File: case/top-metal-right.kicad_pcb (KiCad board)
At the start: 2 copper layers, 135 x 93.7 mm, 26 parts, among them SW1 SW_PUSH, SW10 SW_PUSH, SW11 SW_PUSH, SW12 SW_PUSH, SW13 SW_PUSH, SW14 SW_PUSH, SW15 SW_PUSH, SW16 SW_PUSH, SW17 SW_PUSH, SW18 SW_PUSH, SW19 SW_PUSH, SW2 SW_PUSH, SW20 SW_PUSH, SW3 SW_PUSH, SW4 SW_PUSH, SW5 SW_PUSH, SW6 SW_PUSH, SW7 SW_PUSH, SW8 SW_PUSH, SW9 SW_PUSH

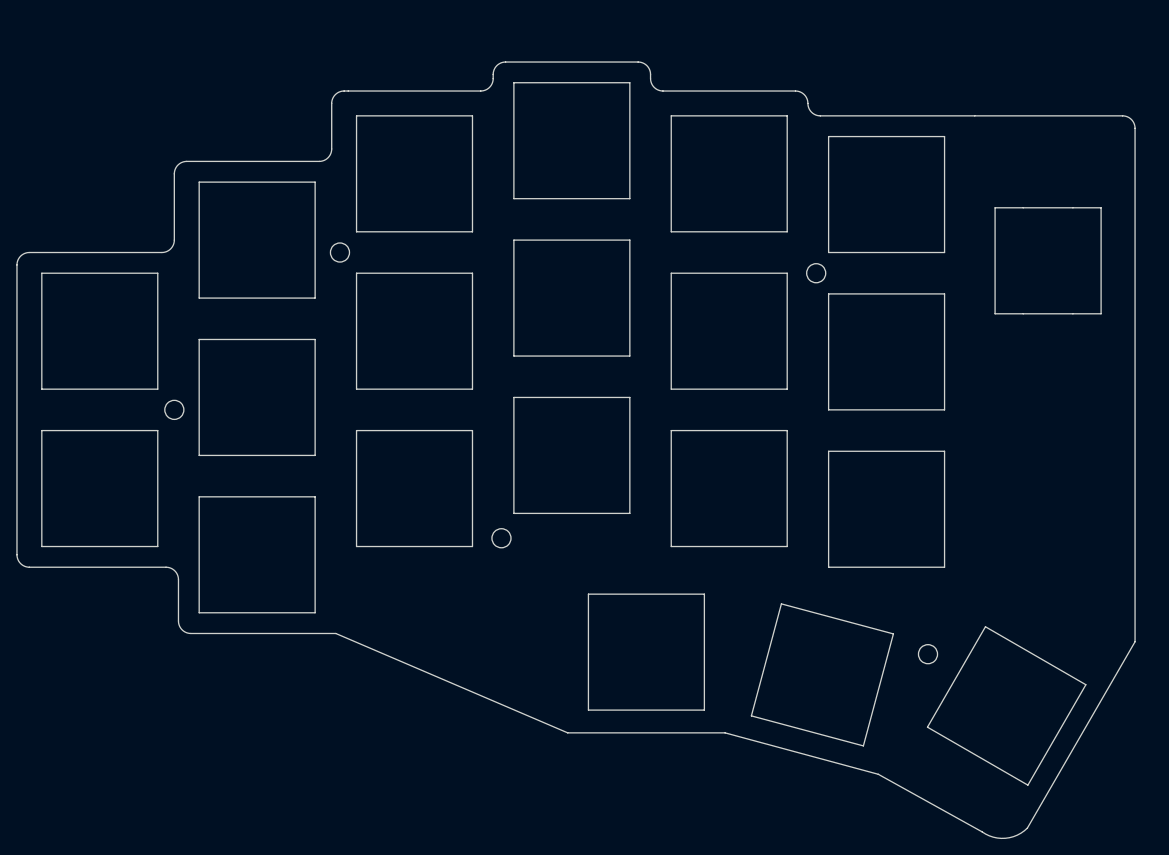
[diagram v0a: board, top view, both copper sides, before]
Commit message: update case files
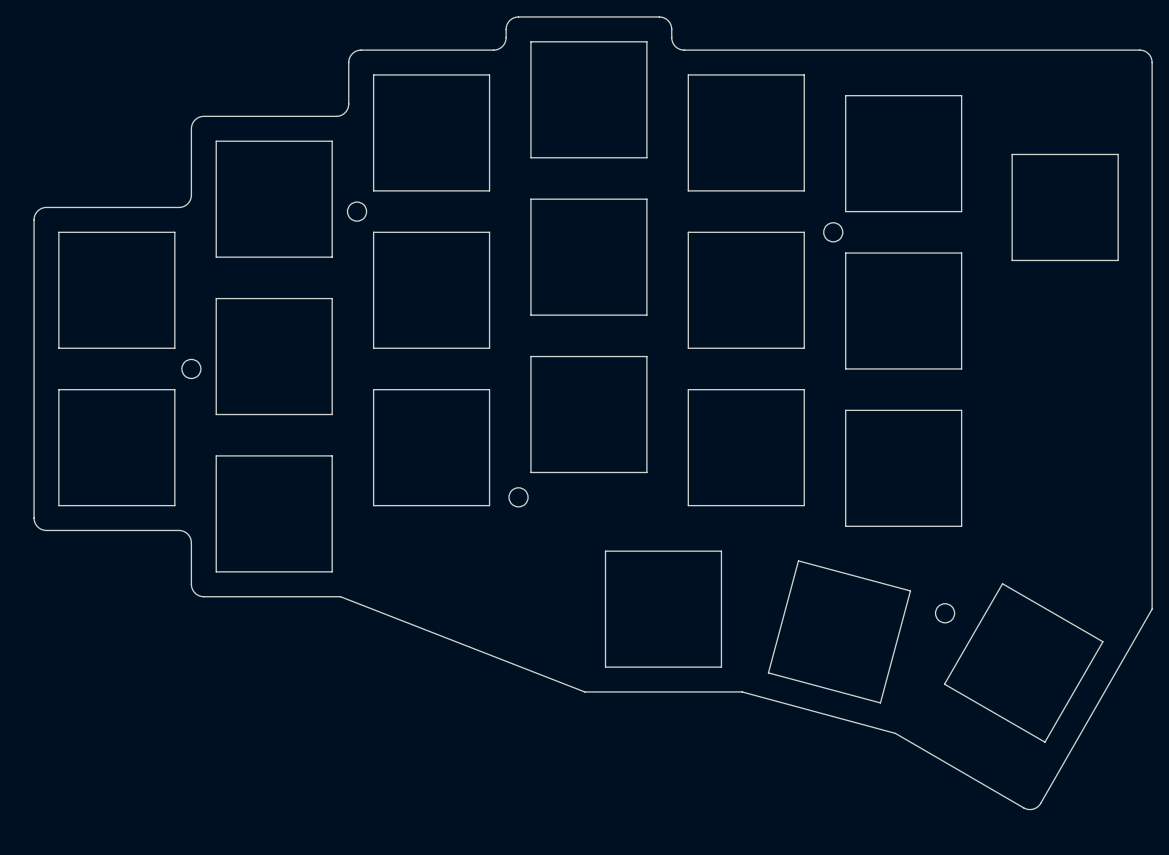
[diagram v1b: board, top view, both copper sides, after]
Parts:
- moved RE1 6.76 mm to (195.1, 69.1)
- moved SW18 5.58 mm to (146.6, 117.6)
- moved SW19 5.58 mm to (167.8, 120.3)
- moved SW20 5.58 mm to (190.1, 124.1)
- moved H2 5.35 mm to (180.6, 118.1)
- moved H4 5.35 mm to (129.1, 104.1)
- moved H5 5.35 mm to (167.1, 72.1)
- moved SW10 5.35 mm to (175.6, 81.6)
- moved SW13 5.35 mm to (137.6, 94.1)
- moved SW14 5.35 mm to (156.6, 98.1)
- moved SW15 5.35 mm to (175.6, 100.6)
- moved SW3 5.35 mm to (137.6, 56.1)
- moved SW4 5.35 mm to (156.6, 60.1)
- moved SW5 5.35 mm to (175.6, 62.6)
- moved SW8 5.35 mm to (137.6, 75.1)
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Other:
- board size 135 x 93.7 mm -> 135 x 95.7 mm
